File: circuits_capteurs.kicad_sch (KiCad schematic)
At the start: 33 parts, among them U2 INA823DT, U3 LMC6482IN, U4 INA823DT, U5 INA823DT

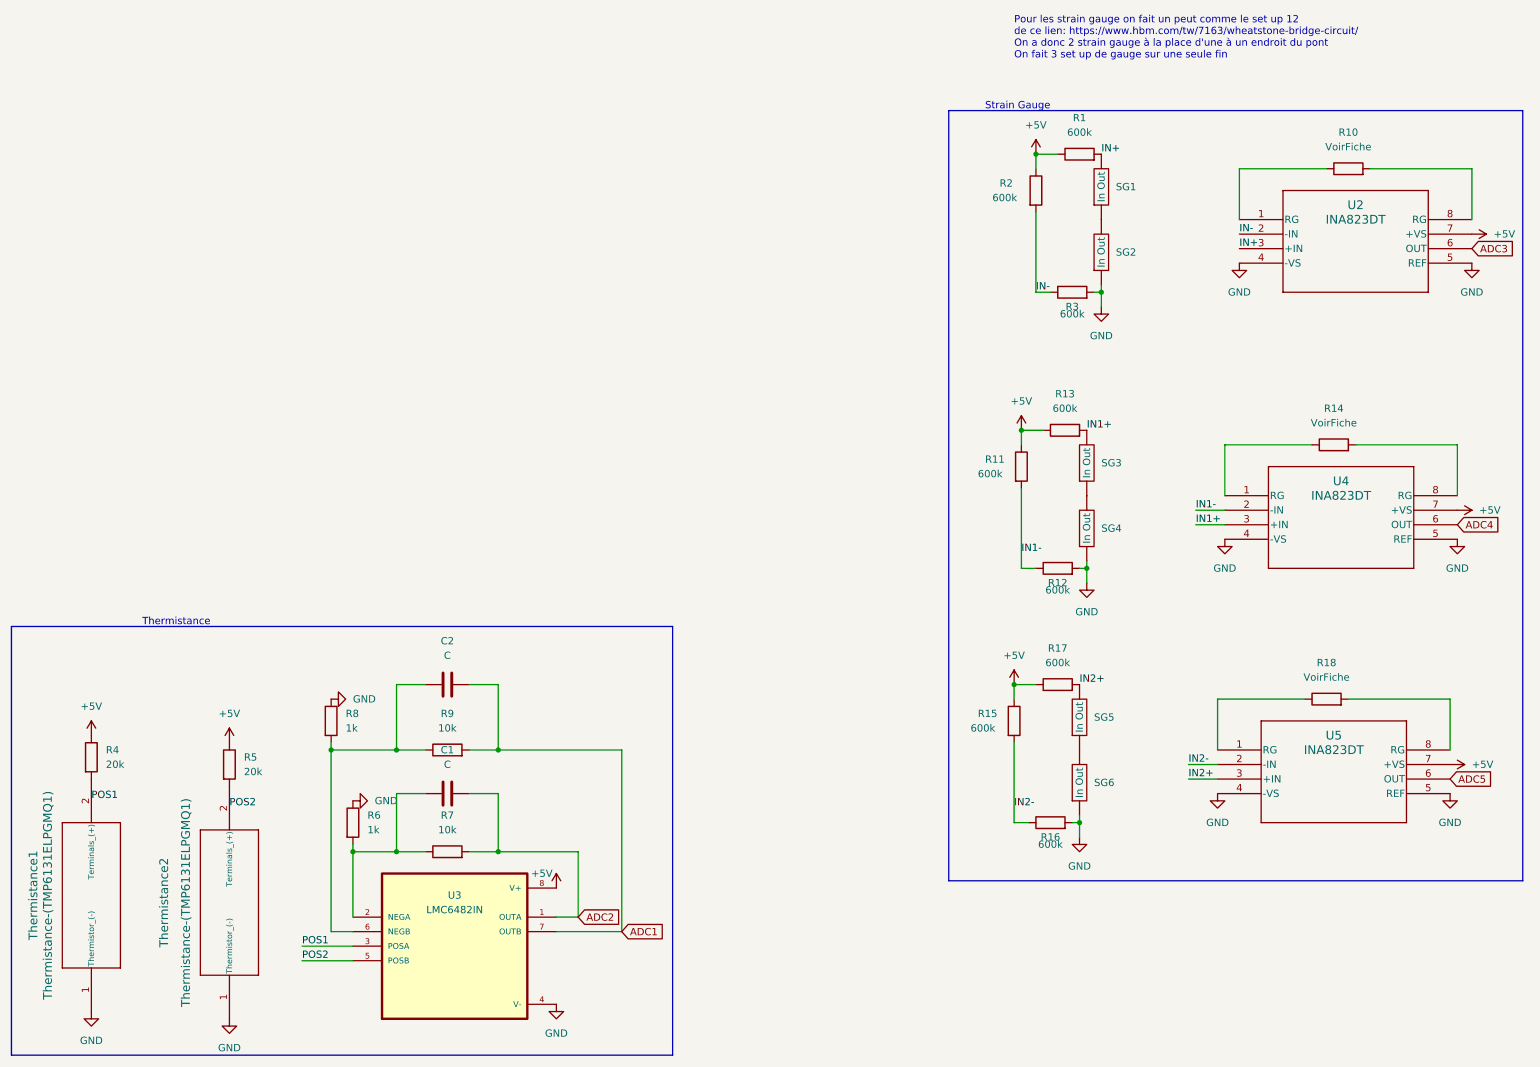
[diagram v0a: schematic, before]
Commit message: LibrairiesFixed
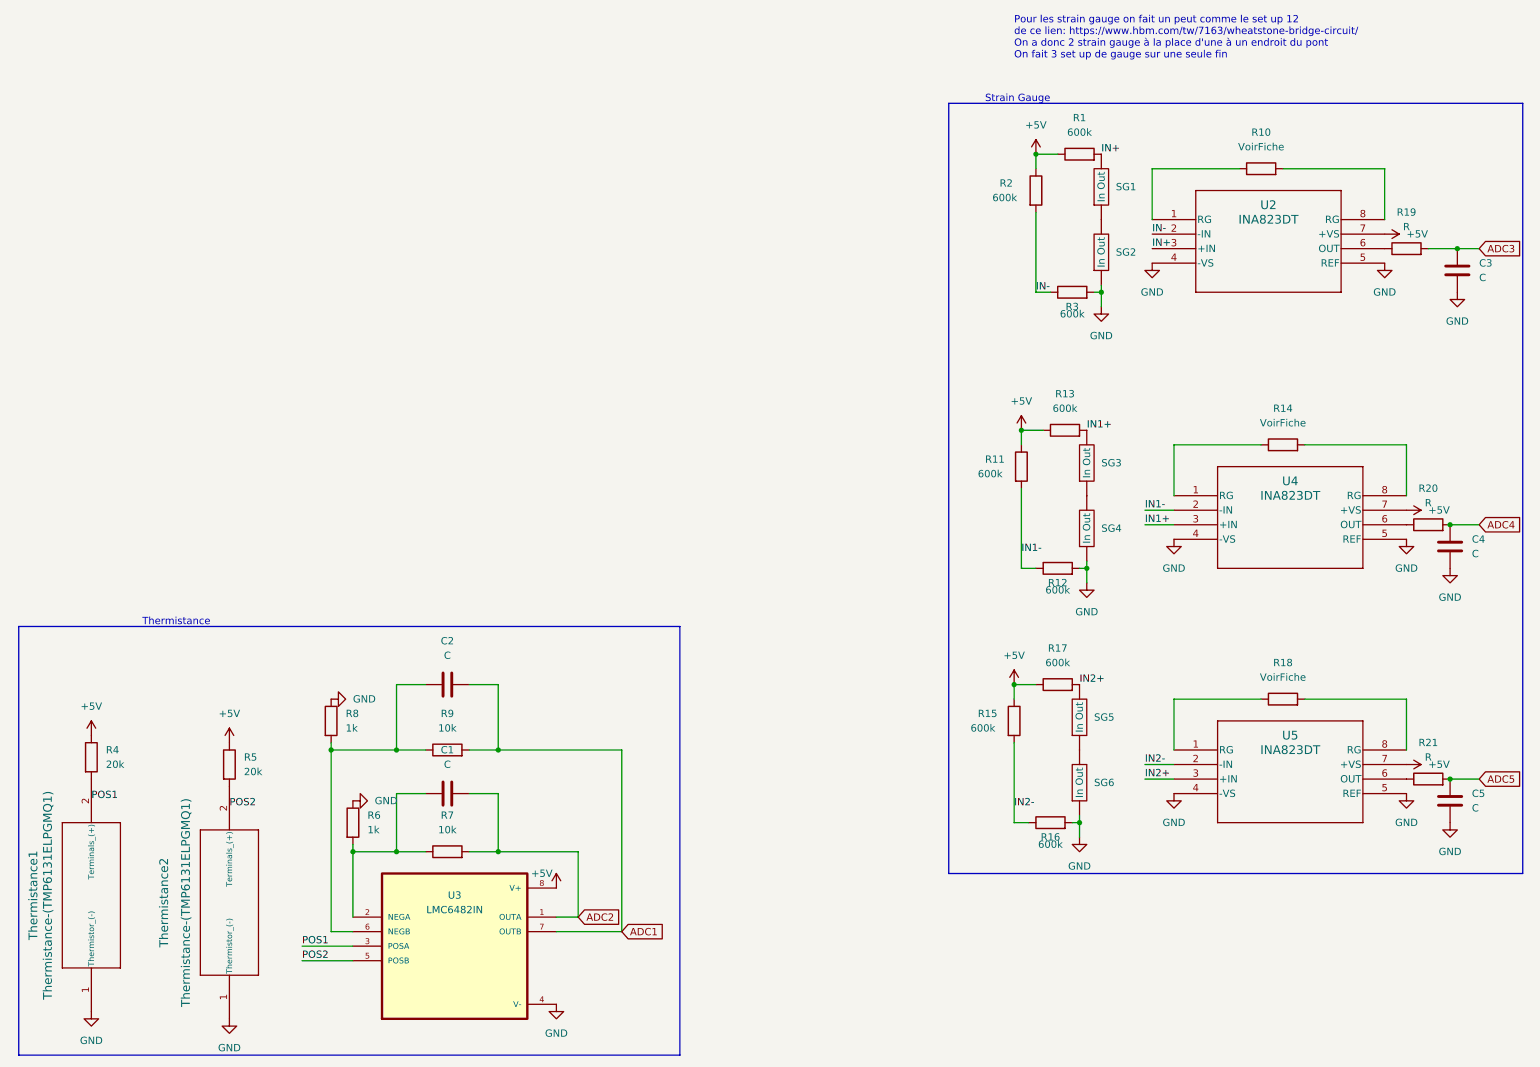
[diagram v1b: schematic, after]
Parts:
- added C3, C4, C5: C, symbol Device:C
- added R19, R20, R21: R, symbol Device:R
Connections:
- net ADC3: now also C3.1, R19.2; no longer U2.6 (OUT)
- net ADC4: now also C4.1, R20.2; no longer U4.6 (OUT)
- net ADC5: now also C5.1, R21.2; no longer U5.6 (OUT)
- net GND: now also C3.2, C4.2, C5.2
- new net: SG1. (Out), SG2. (Out)
- new net: R21.1, U5.6 (OUT)
- new net: R20.1, U4.6 (OUT)
- new net: SG5. (Out), SG6. (Out)
- new net: SG3. (Out), SG4. (Out)
- new net: R19.1, U2.6 (OUT)
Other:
- moved on the sheet: R10, R14, R18, U2, U4, U5

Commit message: Vibrometers
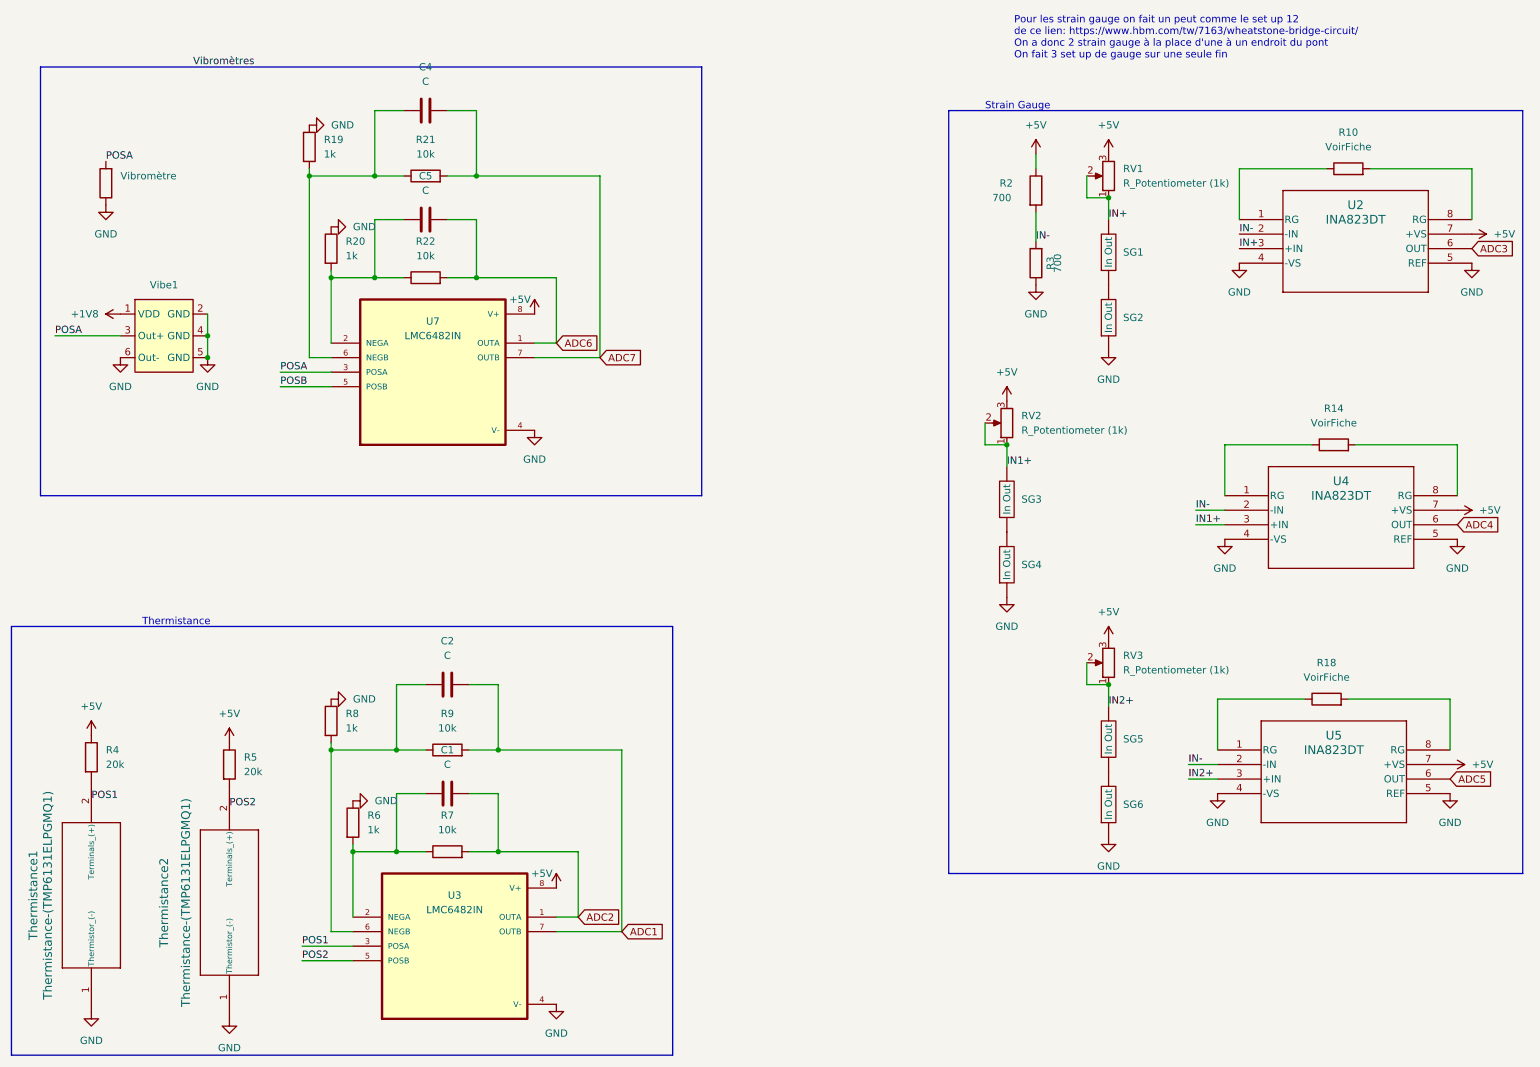
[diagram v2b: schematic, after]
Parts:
- removed C3: C, symbol Device:C
- removed R1, R11, R12, R13, R15, R16, R17: 600k, symbol Device:R
- added R22: 10k, symbol Device:R
- added RV1, RV2, RV3: R_Potentiometer (1k), symbol Device:R_Potentiometer
- added U7: LMC6482IN, LMC6482IN:DIP794W45P254L959H508Q8, symbol GAUL-Symboles:LMC6482IN
- added Vibe1: ~, symbol GAUL-Symboles:Vibromètre_(Surface_Mount)
- added Vibromètre: 1k, symbol Device:R
- R19, R20: value R -> 1k
- R2, R3: value 600k -> 700
- R21: value R -> 10k
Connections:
- net IN1- is gone; now on net IN-: U4.2 (-IN)
- net IN2- is gone; now on net IN-: U5.2 (-IN)
- net +5V: now also RV1.3, RV2.3, RV3.3, U7.8 (V+)
- net ADC3: now also U2.6 (OUT); no longer R19.2
- net ADC4: now also U4.6 (OUT); no longer C4.1, R20.2
- net ADC5: now also U5.6 (OUT); no longer C5.1, R21.2
- net GND: now also R19.1, R20.1, R3.1, U7.4 (V-), Vibe1.2 (GND), Vibe1.4 (GND), Vibe1.5 (GND), Vibe1.6 (Out-), Vibromètre.1; no longer C4.2, C5.2, R3.2
- net IN+: now also RV1.1, RV1.2
- net IN-: now also R3.2; no longer R3.1
- net IN1+: now also RV2.1, RV2.2
- net IN2+: now also RV3.1, RV3.2
- net at R21.1: now also C4.1, R19.2, U7.6 (NEGB); no longer U5.6 (OUT)
- new net: C5.1, R20.2, R22.1, U7.2 (NEGA)
- new net: SG1. (Out), SG2. (Out)
- new net: SG5. (Out), SG6. (Out)
- new net: SG3. (Out), SG4. (Out)
- new net +1V8: Vibe1.1 (VDD)
- new net ADC6: C5.2, R22.2, U7.1 (OUTA)
- new net ADC7: C4.2, R21.2, U7.7 (OUTB)
- new net POSA: U7.3 (POSA), Vibe1.3 (Out+), Vibromètre.2
- new net POSB: U7.5 (POSB)
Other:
- moved on the sheet: R10, R14, R18, R3, SG1, SG2, U2, U4, U5

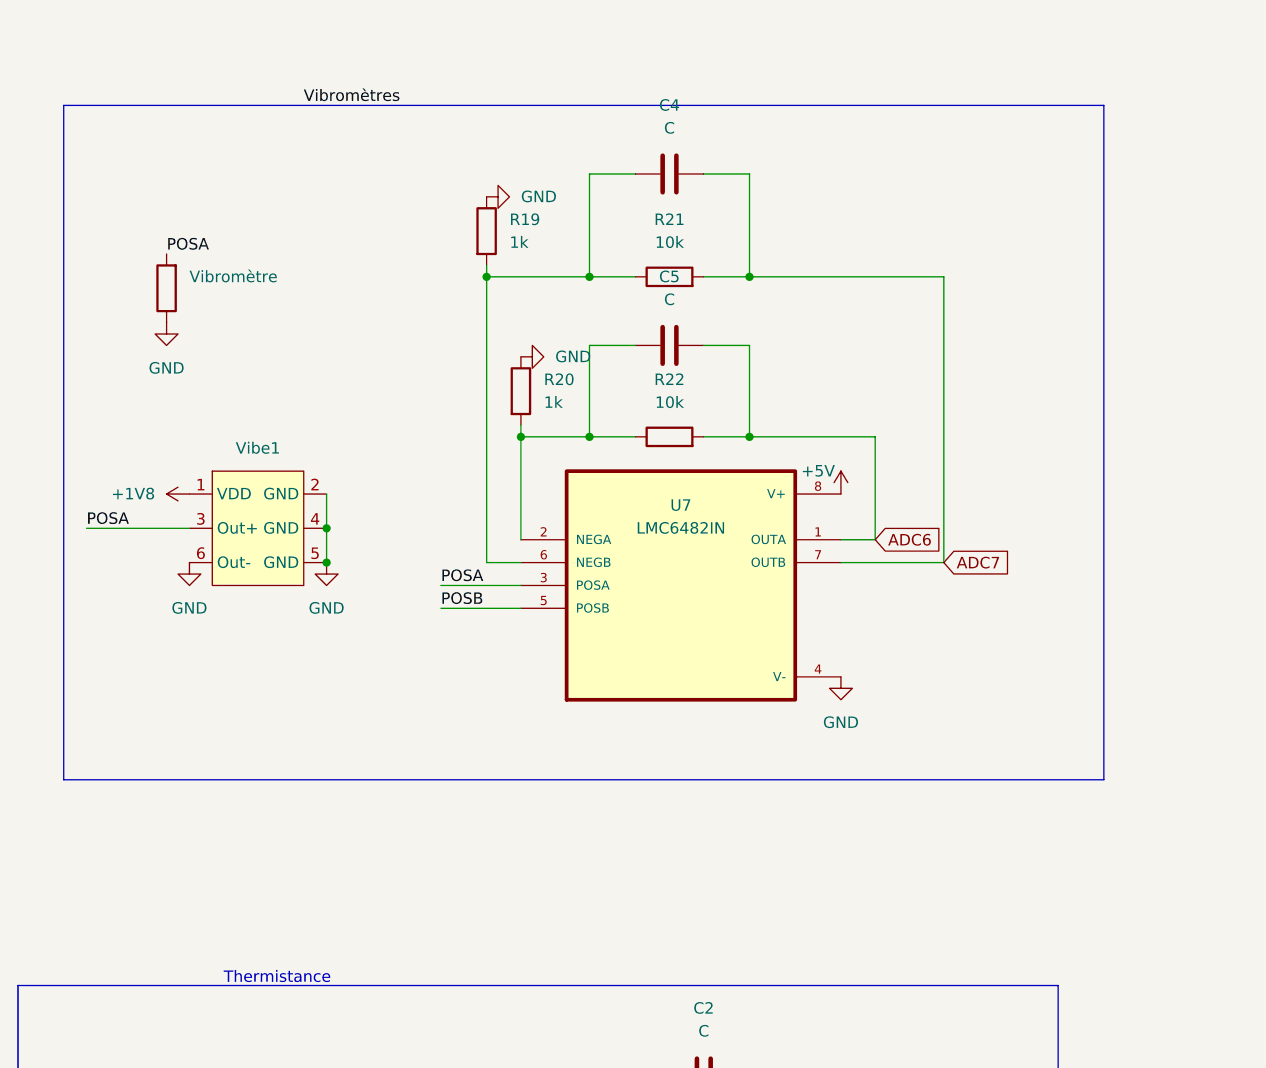
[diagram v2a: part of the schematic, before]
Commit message: Vibing
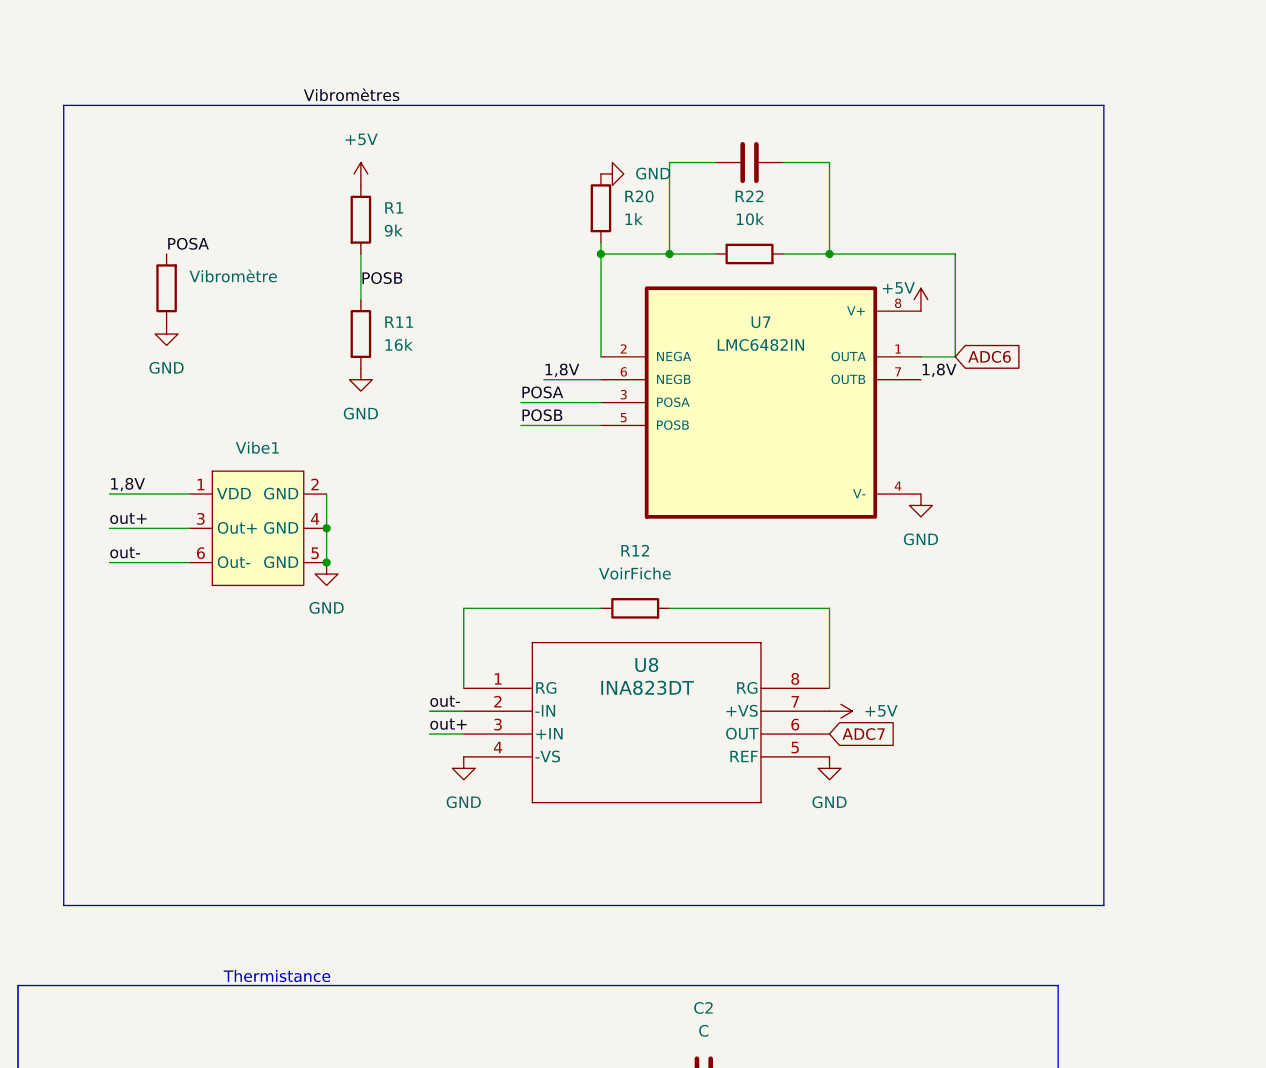
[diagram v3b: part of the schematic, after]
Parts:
- removed C4: C, symbol Device:C
- removed R19: 1k, symbol Device:R
- removed R21: 10k, symbol Device:R
- added R1: 9k, symbol Device:R
- added R11: 16k, symbol Device:R
- added R12: VoirFiche, symbol Device:R
- added U8: INA823DT, D0008A_SOIC_TEX, symbol GAUL-Symboles:INA823DT
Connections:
- net +1V8 is gone; now on net 1,8V: Vibe1.1 (VDD)
- net +5V: now also R1.1, U8.7 (+VS)
- net ADC7: now also U8.6 (OUT); no longer U7.7 (OUTB)
- net GND: now also R11.2, U8.4 (-VS), U8.5 (REF); no longer Vibe1.6 (Out-)
- net POSA: no longer Vibe1.3 (Out+)
- net POSB: now also R1.2, R11.1
- net 1,8V: now reaches U7.6 (NEGB)
- net 1,8V: now also U7.7 (OUTB)
- new net: R12.1, U8.1 (RG)
- new net: R12.2, U8.8 (RG)
- new net: SG1. (Out), SG2. (Out)
- new net: SG5. (Out), SG6. (Out)
- new net: SG3. (Out), SG4. (Out)
- new net out+: U8.3 (+IN), Vibe1.3 (Out+)
- new net out-: U8.2 (-IN), Vibe1.6 (Out-)
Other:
- moved on the sheet: R20, R22, U7
